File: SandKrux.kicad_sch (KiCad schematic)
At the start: 101 parts, among them CN1 527450697, J1 Conn_01x02, Q1 S8050, Q2 SI2301CDS-T1-GE3, U1 K210_C913414, U2 AXP173, U3 MT9700-N, U4 XC6206P182MR_C347373, U5 GD25LQ128EWIGR, U6 TMI7003C, U7 SGM803-TXN3/TR_C5152602, U8 XC6206P302MR_C347375, X1 X322526MMB4SI

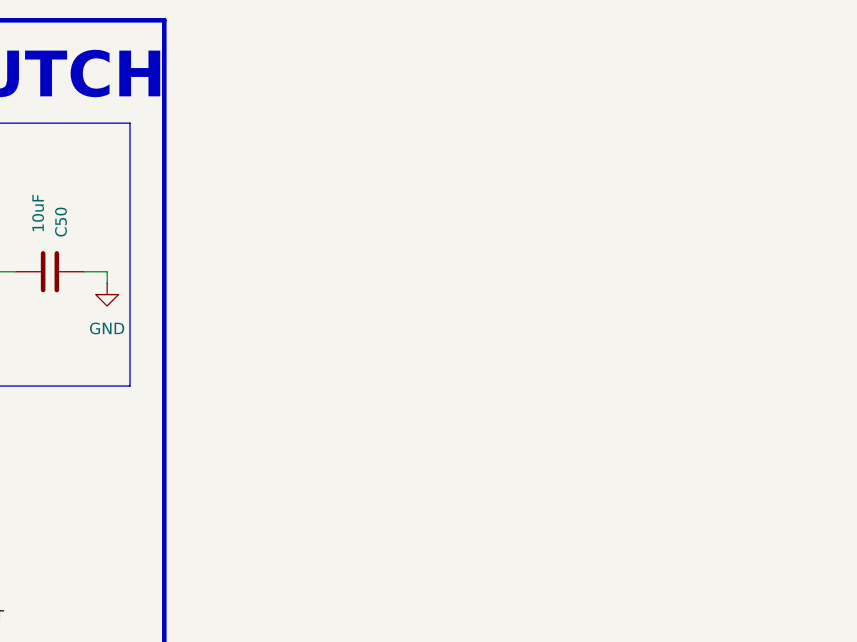
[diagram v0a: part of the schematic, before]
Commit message: TFT CARD
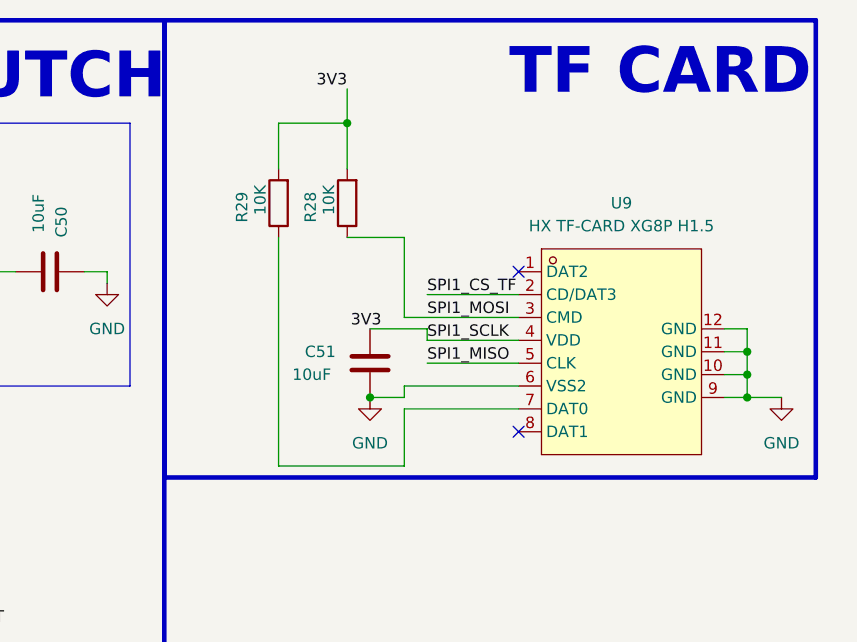
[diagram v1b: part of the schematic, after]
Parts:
- added C51: 10uF, Capacitor_SMD:C_0201_0603Metric, symbol Device:C
- added R28, R29: 10K, Resistor_SMD:R_0201_0603Metric, symbol Device:R
- added U9: HX TF-CARD XG8P H1.5, easyeda2kicad:TF-SMD_HX-TF-CARD-XG8P-H1.5, symbol easyeda2kicad:HXTF-CARDXG8PH1.5
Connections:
- net GND: now also C51.1, U9.10 (GND), U9.11 (GND), U9.12 (GND), U9.6 (VSS2), U9.9 (GND)
- net at C37.1, C4.2, C49.1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: now also C51.2, R28.2, R29.2, U9.4 (VDD)
- new net: R29.1, U9.7 (DAT0)
- new net SPI1_CS_TF: U9.2 (CD/DAT3)
- new net SPI1_MISO: U9.5 (CLK)
- new net SPI1_MOSI: R28.1, U9.3 (CMD)
- no-connect marks 70 -> 72
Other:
- note added: "TF CARD"

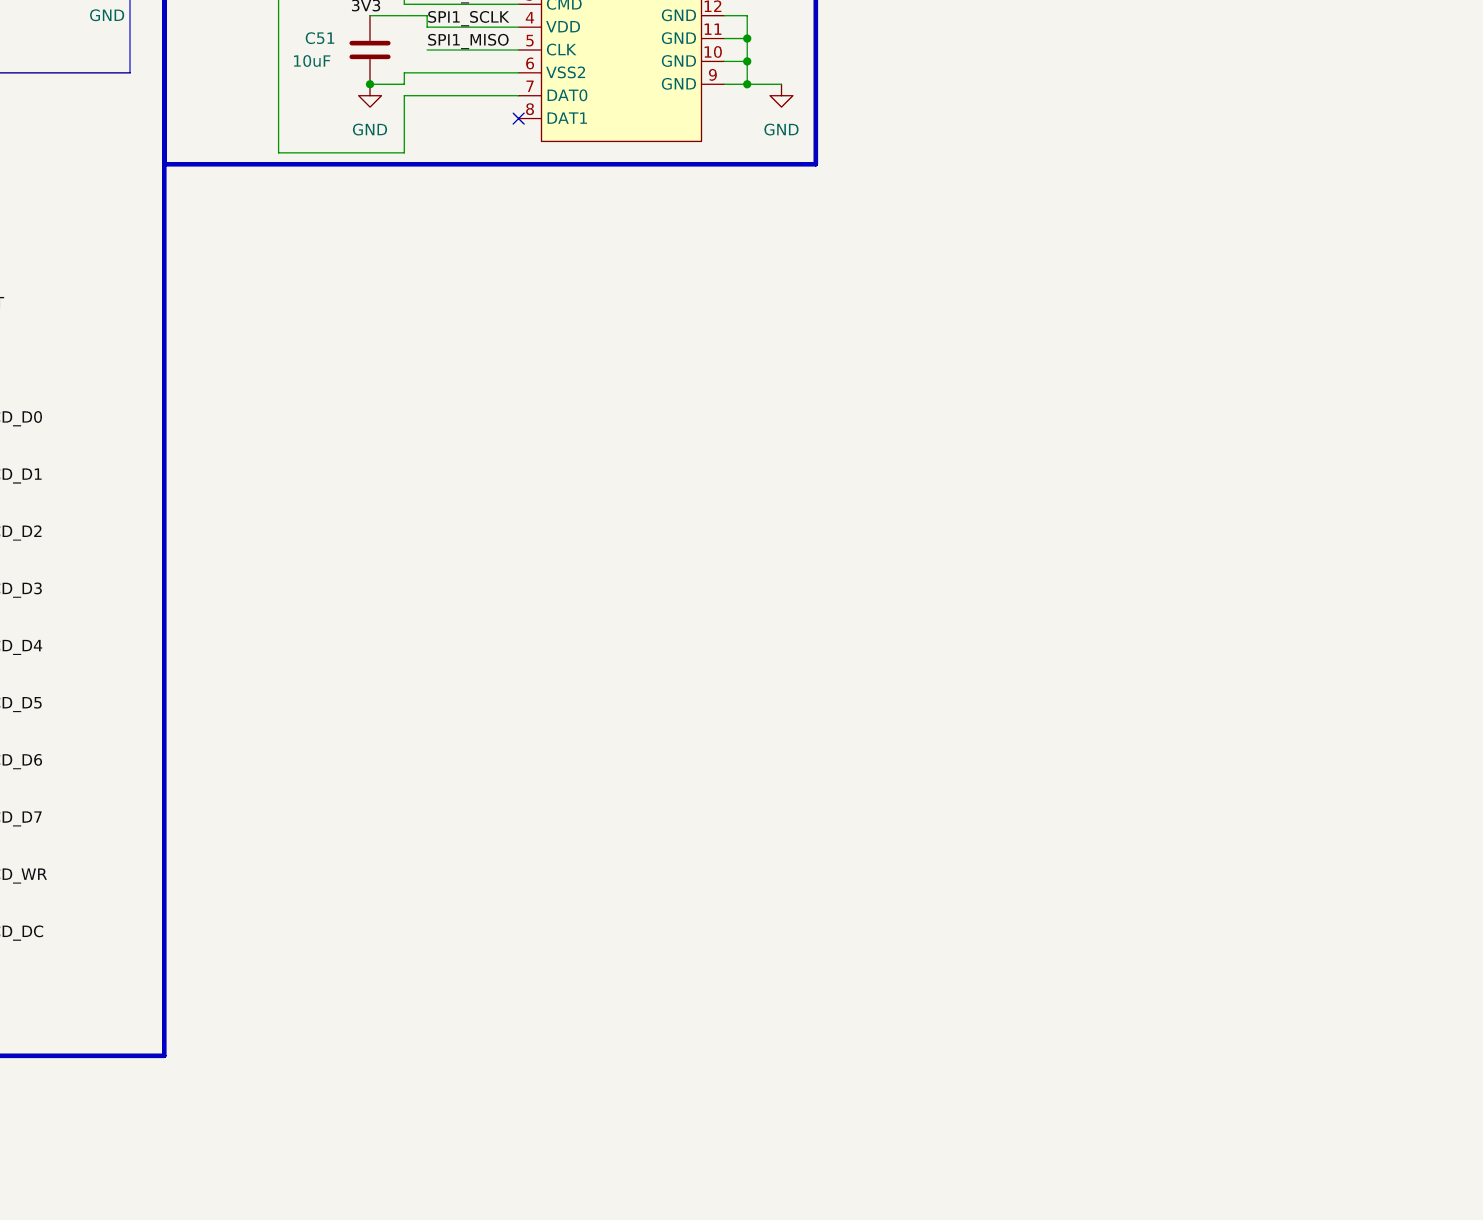
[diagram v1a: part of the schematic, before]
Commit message: usb ports
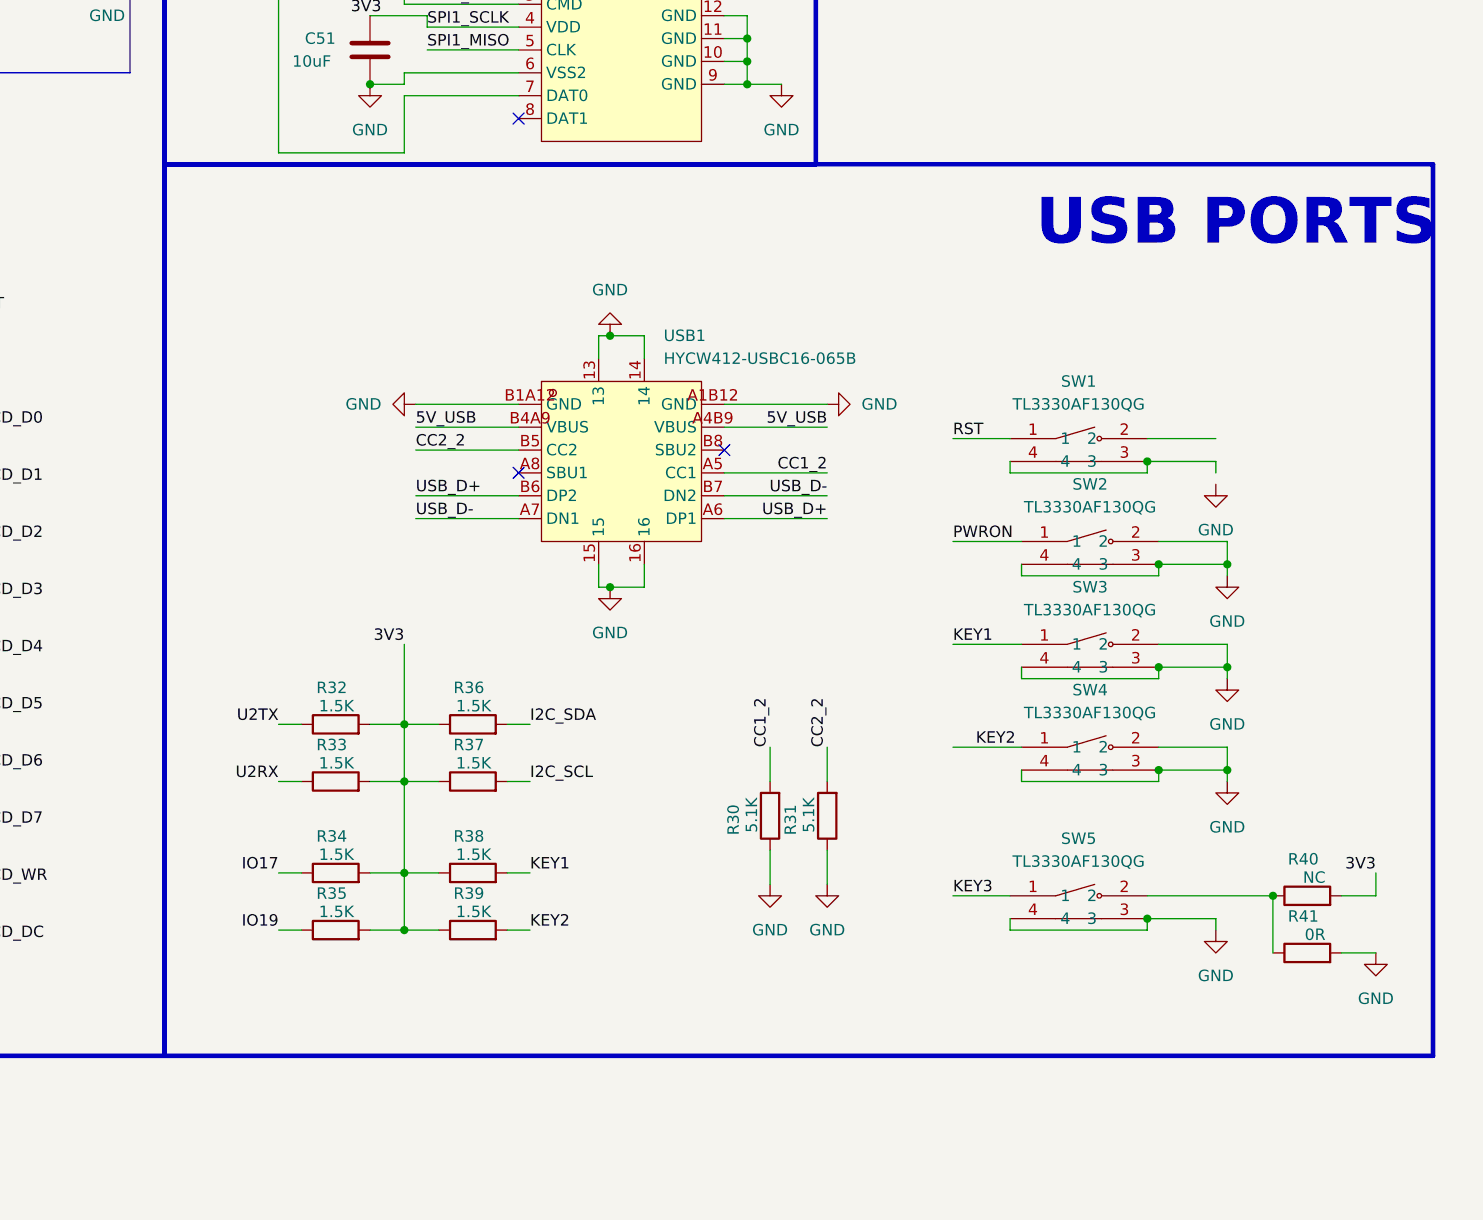
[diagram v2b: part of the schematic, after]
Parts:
- added R30, R31: 5.1K, Resistor_SMD:R_0201_0603Metric, symbol Device:R
- added R32, R33, R34, R35, R36, R37, R38, R39: 1.5K, Resistor_SMD:R_0201_0603Metric, symbol Device:R
- added R40: NC, Resistor_SMD:R_0201_0603Metric, symbol Device:R
- added R41: 0R, Resistor_SMD:R_0201_0603Metric, symbol Device:R
- added SW1, SW2, SW3, SW4, SW5: TL3330AF130QG, easyeda2kicad:SW-SMD_E-SWITCH_TL3330, symbol easyeda2kicad:TL3330AF130QG
- added USB1: HYCW412-USBC16-065B, easyeda2kicad:USB-C-SMD_HYCW412-USBC16-065B, symbol easyeda2kicad:HYCW412-USBC16-065B
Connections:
- net GND: now also R30.1, R31.1, R41.2, SW2.2, SW2.3, SW2.4, SW3.2, SW3.3, SW3.4, SW4.2, SW4.3, SW4.4, SW5.3, SW5.4, USB1.13, USB1.14, USB1.15, USB1.16, USB1.A1B12 (GND), USB1.B1A12 (GND)
- net I2C_SCL: now also R37.2
- net I2C_SDA: now also R36.2
- net RST: now also SW1.1
- net at C37.1, C4.2, C49.1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: now also R32.2, R33.2, R34.2, R35.2, R36.1, R37.1, R38.1, R39.1, R40.2
- new net: R40.1, R41.1, SW5.2
- new net: SW1.3, SW1.4
- new net 5V_USB: USB1.A4B9 (VBUS), USB1.B4A9 (VBUS)
- new net CC1_2: R30.2, USB1.A5 (CC1)
- new net CC2_2: R31.2, USB1.B5 (CC2)
- new net IO17: R34.1
- new net IO19: R35.1
- new net KEY1: R38.2, SW3.1
- new net KEY2: R39.2, SW4.1
- new net KEY3: SW5.1
- new net PWRON: SW2.1
- new net U2RX: R33.1
- new net U2TX: R32.1
- new net USB_D+: USB1.A6 (DP1), USB1.B6 (DP2)
- new net USB_D-: USB1.A7 (DN1), USB1.B7 (DN2)
- no-connect marks 72 -> 74
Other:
- note added: "USB PORTS"
